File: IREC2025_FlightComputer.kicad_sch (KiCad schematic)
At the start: 69 parts, among them J1 Molex Microfit, J2 BOOT0, J3 Companion, J5 SWD, Q1 SI7232DN-T1-GE3, U1 STM32U575VGTx, U13 TLV75733PDBV, U8 TPS62153, U9 SN74HCT125DR, X1 1XXD32000MBA

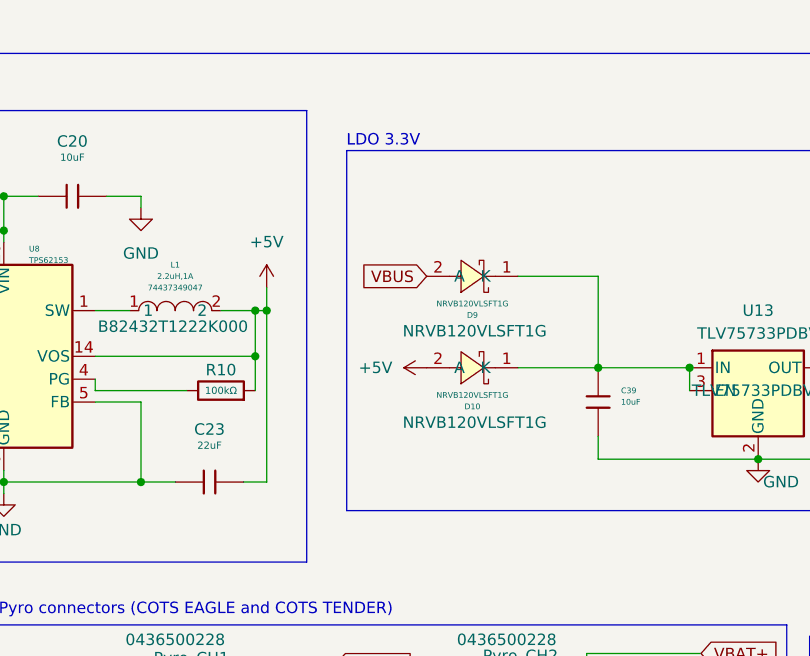
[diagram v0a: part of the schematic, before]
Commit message: adjustments
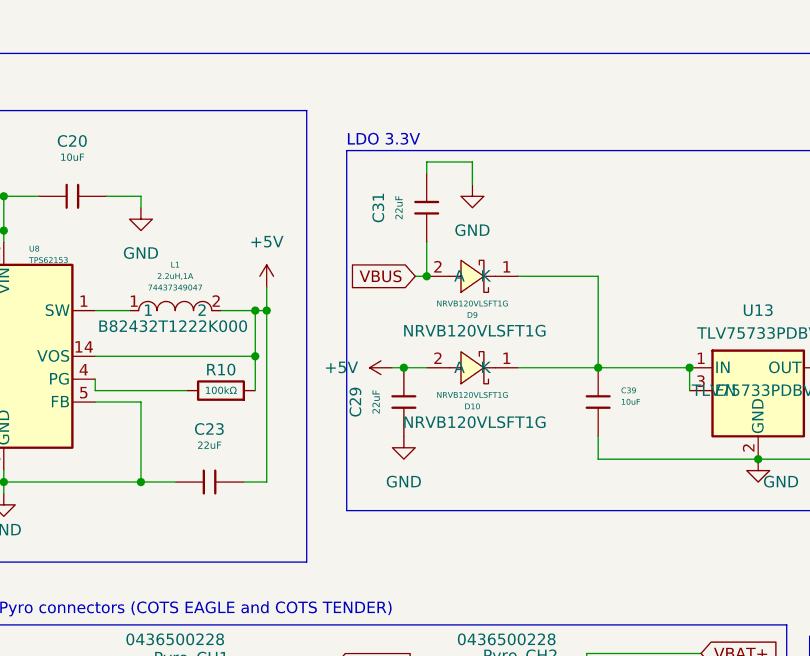
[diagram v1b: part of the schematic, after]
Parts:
- added C29, C31: 22uF, PCM_JLCPCB:C_0603, symbol PCM_JLCPCB-Capacitors:0603,22uF
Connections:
- net +5V: now also C29.2
- net GND: now also C29.1, C31.2
- net VBUS: now also C31.1
